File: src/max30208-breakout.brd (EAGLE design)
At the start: 13 x 7.8 mm, 4 parts, among them J1 PTH VERT MALE, J2 PTH VERT MALE, U1 MAX30208CLB+T

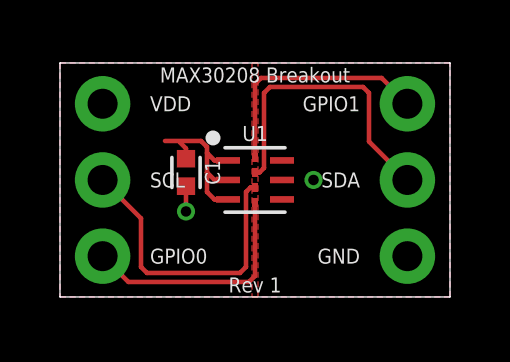
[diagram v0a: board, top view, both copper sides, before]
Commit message: Update CAM files.
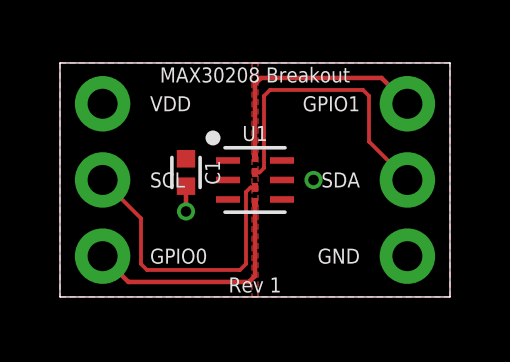
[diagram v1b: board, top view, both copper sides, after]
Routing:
- net VDD: track 6.02 -> 0.00 mm
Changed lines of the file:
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@@
 <setting verticaltext="up"/>
 </settings>
-<grid distance="1" unitdist="mm" unit="mm" style="lines" multiple="1" display="yes" altdistance="0.1" altunitdist="mm" altunit="mm"/>
+<grid distance="0.1" unitdist="mm" unit="mm" style="lines" multiple="1" display="yes" altdistance="0.05" altunitdist="mm" altunit="mm"/>
 <layers>
 <layer number="1" name="Top" color="4" fill="1" visible="yes" active="yes"/>
@@
 </class>
 </classes>
-<designrules name="stella-wearables">
-<description language="en">&lt;b&gt;Stella Wearables Design Rules based on OSH Park Design Rules&lt;/b&gt;
+<designrules name="oshpark-2layer">
+<description language="en">&lt;b&gt;OSH Park Design Rules&lt;/b&gt;
 &lt;p&gt;
 Please make sure your boards conform to these design rules.
@@
 <param name="mtCopper" value="0.035559375mm 0.0356mm 0.0356mm 0.0356mm 0.0356mm 0.0356mm 0.0356mm 0.0356mm 0.0356mm 0.0356mm 0.0356mm 0.0356mm 0.0356mm 0.0356mm 0.0356mm 0.035559375mm"/>
 <param name="mtIsolate" value="1.6mm 0.1499mm 0.2007mm 0.1499mm 0.2007mm 0.1499mm 0.2007mm 0.1499mm 0.2007mm 0.1499mm 0.2007mm 0.1499mm 0.2007mm 0.1499mm 0.2007mm"/>
-<param name="mdWireWire" value="3mil"/>
-<param name="mdWirePad" value="3mil"/>
-<param name="mdWireVia" value="3mil"/>
-<param name="mdPadPad" value="3mil"/>
-<param name="mdPadVia" value="3mil"/>
-<param name="mdViaVia" value="3mil"/>
-<param name="mdSmdPad" value="3mil"/>
-<param name="mdSmdVia" value="3mil"/>
-<param name="mdSmdSmd" value="3mil"/>
+<param name="mdWireWire" value="6mil"/>
+<param name="mdWirePad" value="6mil"/>
+<param name="mdWireVia" value="6mil"/>
+<param name="mdPadPad" value="6mil"/>
+<param name="mdPadVia" value="6mil"/>
+<param name="mdViaVia" value="6mil"/>
+<param name="mdSmdPad" value="6mil"/>
+<param name="mdSmdVia" value="6mil"/>
+<param name="mdSmdSmd" value="6mil"/>
 <param name="mdViaViaSameLayer" value="8mil"/>
 <param name="mnLayersViaInSmd" value="2"/>
@@
 <param name="mdDrill" value="6mil"/>
 <param name="mdSmdStop" value="0mil"/>
-<param name="msWidth" value="3mil"/>
-<param name="msDrill" value="6mil"/>
+<param name="msWidth" value="6mil"/>
+<param name="msDrill" value="10mil"/>
 <param name="msMicroVia" value="10mil"/>
 <param name="msBlindViaRatio" value="0.5"/>
@@
 <contactref element="J1" pad="2"/>
 <contactref element="U1" pad="9"/>
-<wire x1="0" y1="-0.25" x2="-0.15" y2="-0.25" width="0.1524" layer="1"/>
-<wire x1="-0.15" y1="-0.25" x2="-0.3" y2="-0.4" width="0.1524" layer="1"/>
-<wire x1="-0.3" y1="-2.9" x2="-0.5" y2="-3.1" width="0.1524" layer="1"/>
-<wire x1="-0.3" y1="-0.4" x2="-0.3" y2="-2.9" width="0.1524" layer="1"/>
-<wire x1="-3.6" y1="-3.1" x2="-3.8" y2="-2.9" width="0.1524" layer="1"/>
-<wire x1="-3.8" y1="-1.28" x2="-5.08" y2="0" width="0.1524" layer="1"/>
-<wire x1="-0.5" y1="-3.1" x2="-3.6" y2="-3.1" width="0.1524" layer="1"/>
-<wire x1="-3.8" y1="-2.9" x2="-3.8" y2="-1.28" width="0.1524" layer="1"/>
+<wire x1="0" y1="-0.25" x2="-0.15" y2="-0.25" width="0.127" layer="1"/>
+<wire x1="-0.3" y1="-0.4" x2="-0.15" y2="-0.25" width="0.127" layer="1"/>
+<wire x1="-0.3" y1="-2.8" x2="-0.5" y2="-3" width="0.127" layer="1"/>
+<wire x1="-0.3" y1="-0.4" x2="-0.3" y2="-2.8" width="0.127" layer="1"/>
+<wire x1="-3.6" y1="-3" x2="-3.8" y2="-2.8" width="0.127" layer="1"/>
+<wire x1="-3.8" y1="-1.28" x2="-5.08" y2="0" width="0.127" layer="1"/>
+<wire x1="-0.5" y1="-3" x2="-3.6" y2="-3" width="0.127" layer="1"/>
+<wire x1="-3.8" y1="-2.8" x2="-3.8" y2="-1.28" width="0.127" layer="1"/>
 </signal>
 <signal name="SDA">
 <contactref element="U1" pad="8"/>
-<wire x1="0" y1="0.25" x2="0.15" y2="0.25" width="0.1524" layer="1"/>
-<wire x1="0.15" y1="0.25" x2="0.3" y2="0.4" width="0.1524" layer="1"/>
+<wire x1="0" y1="0.25" x2="0.15" y2="0.25" width="0.127" layer="1"/>
+<wire x1="0.15" y1="0.25" x2="0.3" y2="0.4" width="0.127" layer="1"/>
 <contactref element="J2" pad="2"/>
-<wire x1="0.3" y1="0.4" x2="0.3" y2="2.9" width="0.1524" layer="1"/>
-<wire x1="0.3" y1="2.9" x2="0.5" y2="3.1" width="0.1524" layer="1"/>
-<wire x1="0.5" y1="3.1" x2="3.6" y2="3.1" width="0.1524" layer="1"/>
-<wire x1="3.6" y1="3.1" x2="3.8" y2="2.9" width="0.1524" layer="1"/>
-<wire x1="3.8" y1="1.28" x2="5.08" y2="0" width="0.1524" layer="1"/>
-<wire x1="3.8" y1="2.9" x2="3.8" y2="1.28" width="0.1524" layer="1"/>
+<wire x1="0.3" y1="0.4" x2="0.3" y2="2.8" width="0.127" layer="1"/>
+<wire x1="0.3" y1="2.8" x2="0.5" y2="3" width="0.127" layer="1"/>
+<wire x1="0.5" y1="3" x2="3.6" y2="3" width="0.127" layer="1"/>
+<wire x1="3.6" y1="3" x2="3.8" y2="2.8" width="0.127" layer="1"/>
+<wire x1="3.8" y1="1.28" x2="5.08" y2="0" width="0.127" layer="1"/>
+<wire x1="3.8" y1="2.8" x2="3.8" y2="1.28" width="0.127" layer="1"/>
 </signal>
 <signal name="VDD">
@@
 <contactref element="U1" pad="1"/>
 <contactref element="C1" pad="1"/>
-<wire x1="-0.9" y1="0" x2="-1.35" y2="0" width="0.1524" layer="1"/>
-<wire x1="-1.35" y1="0" x2="-1.6" y2="0.25" width="0.1524" layer="1"/>
-<wire x1="-1.6" y1="0.25" x2="-1.6" y2="0.9" width="0.1524" layer="1"/>
-<wire x1="-1.6" y1="0.9" x2="-1.6" y2="1.1" width="0.1524" layer="1"/>
-<wire x1="-0.9" y1="-0.65" x2="-1.35" y2="-0.65" width="0.1524" layer="1"/>
-<wire x1="-1.35" y1="-0.65" x2="-1.6" y2="-0.4" width="0.1524" layer="1"/>
-<wire x1="-1.6" y1="-0.4" x2="-1.6" y2="0.25" width="0.1524" layer="1"/>
-<wire x1="-0.9" y1="0.65" x2="-1.35" y2="0.65" width="0.1524" layer="1"/>
-<wire x1="-1.35" y1="0.65" x2="-1.6" y2="0.9" width="0.1524" layer="1"/>
-<wire x1="-1.6" y1="1.1" x2="-1.8" y2="1.3" width="0.1524" layer="1"/>
-<wire x1="-1.8" y1="1.3" x2="-3" y2="1.3" width="0.1524" layer="1"/>
-<wire x1="-2.3" y1="0.7075" x2="-2.3" y2="1.05" width="0.1524" layer="1"/>
-<wire x1="-2.3" y1="1.05" x2="-2.5" y2="1.25" width="0.1524" layer="1"/>
 <contactref element="J1" pad="1"/>
 </signal>
